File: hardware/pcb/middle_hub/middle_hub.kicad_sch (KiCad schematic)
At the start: 16 parts, among them J1 USB_A, J2 FH34SRJ-12S-0.5SH, J3 FH34SRJ-12S-0.5SH, J4 Conn_01x05, SW1 RotaryEncoder_Switch, U1 DT1446-04S, U2 AP2112K-3.3

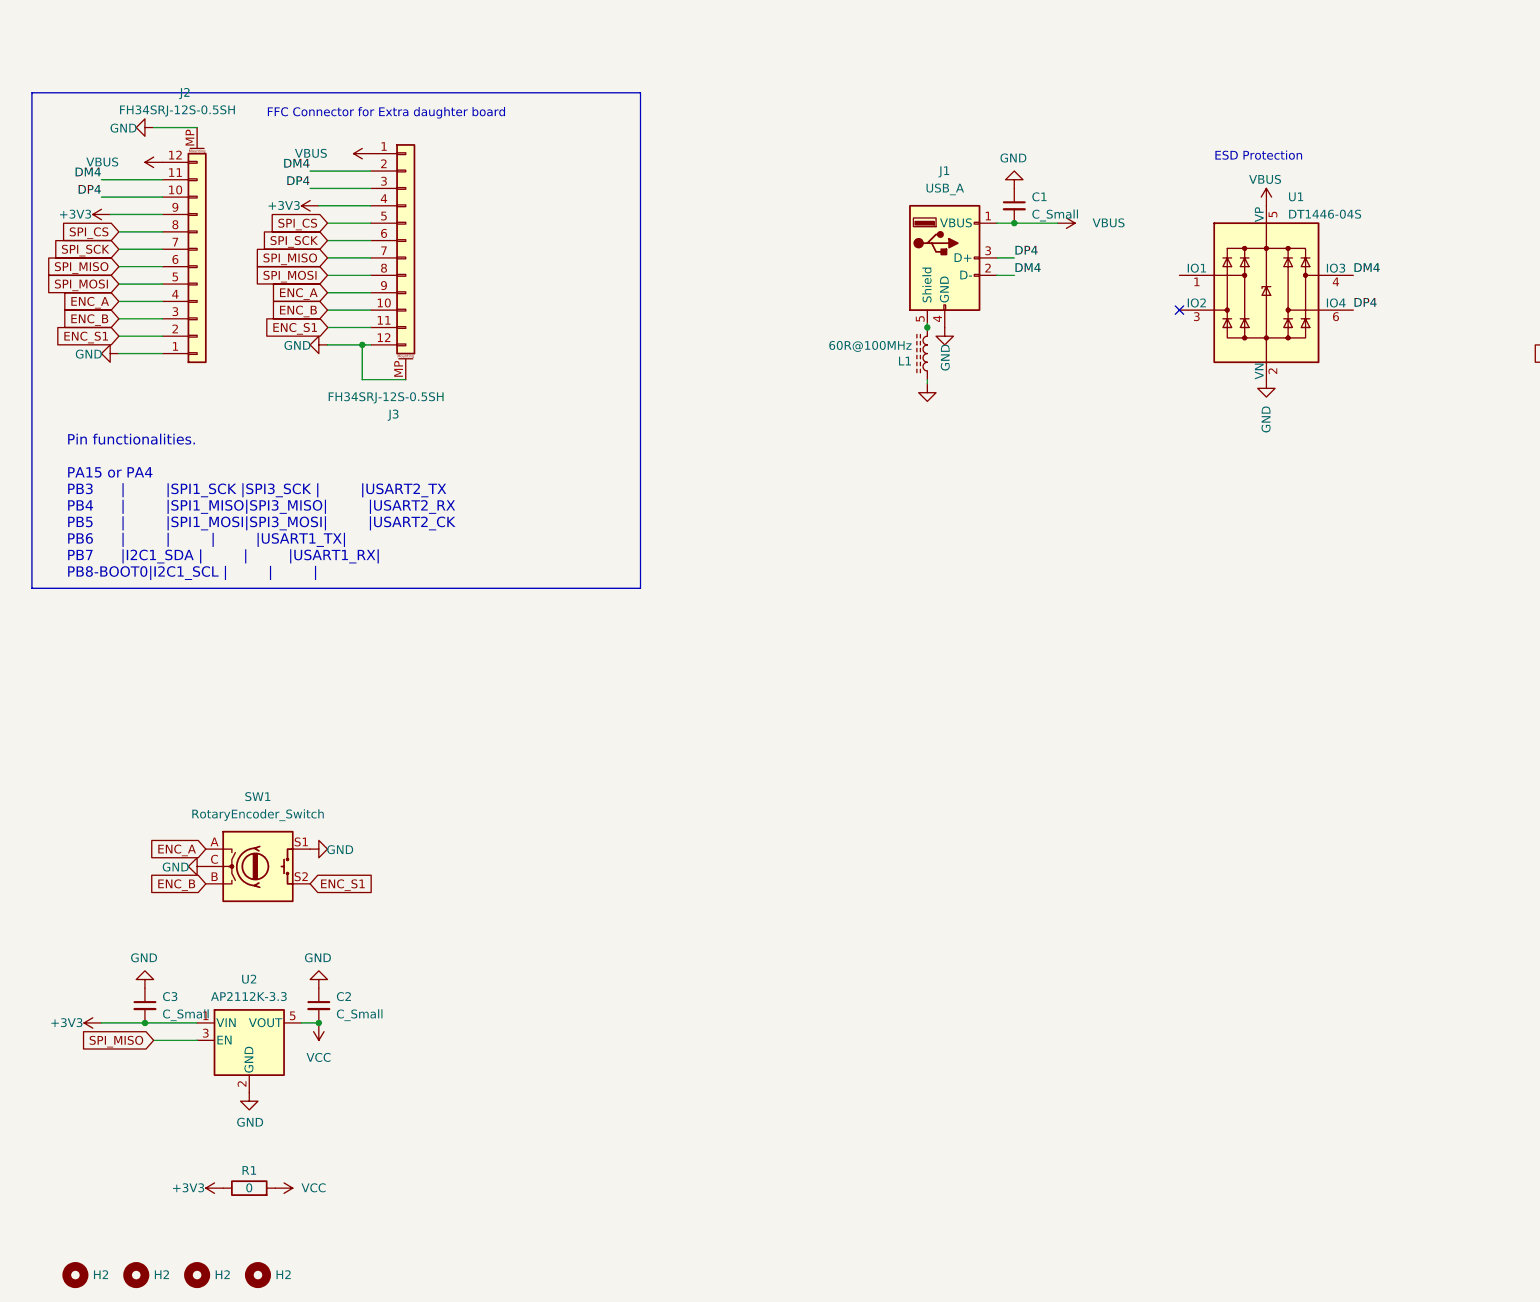
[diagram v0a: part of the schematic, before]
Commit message: preproduction
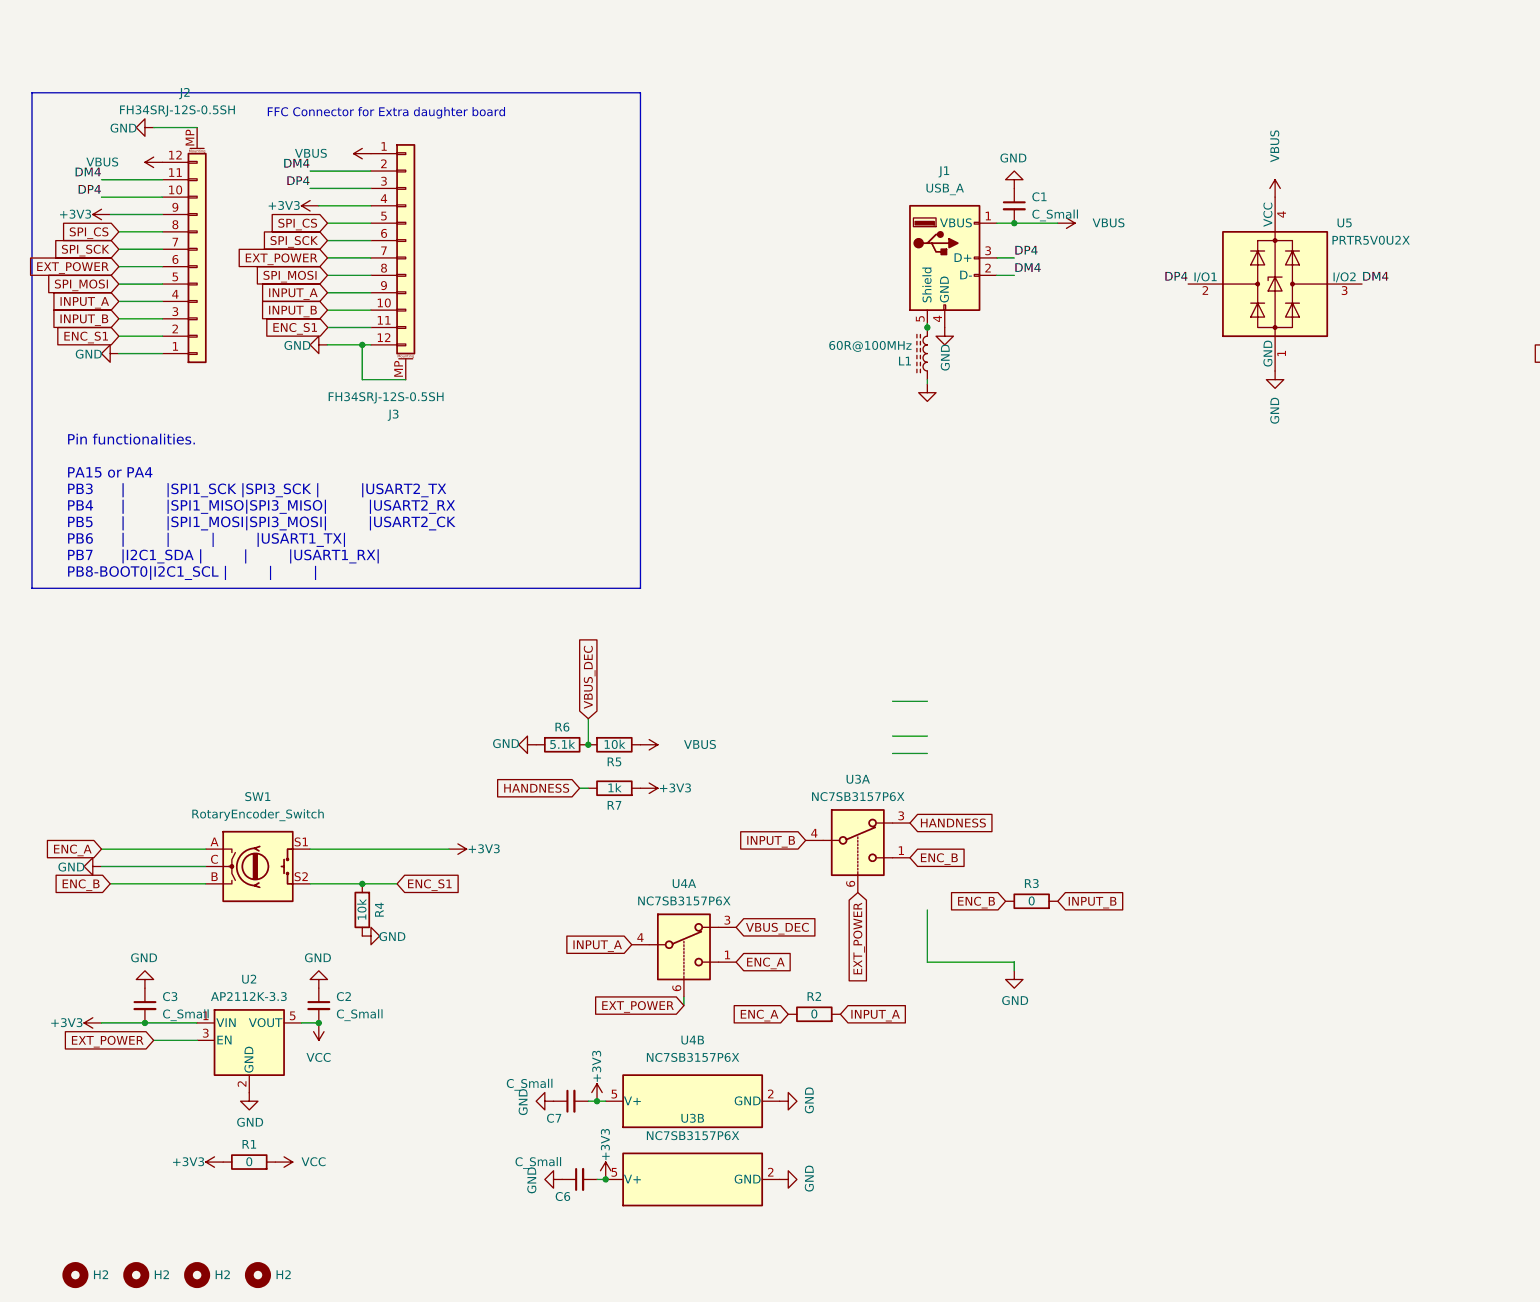
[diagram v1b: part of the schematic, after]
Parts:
- removed U1: DT1446-04S, PCM_Package_TO_SOT_SMD_AKL:SOT-363_SC-70-6_Handsoldering, symbol Power_Protection:SRV05-4
- added C6, C7: C_Small, PCM_Capacitor_SMD_AKL:C_0603_1608Metric_Pad1.05x0.95mm, symbol Device:C_Small
- added R2, R3: 0, PCM_Resistor_SMD_AKL:R_0402_1005Metric_Pad0.72x0.64mm_HandSolder, symbol Device:R
- added R4, R5: 10k, PCM_Resistor_SMD_AKL:R_0603_1608Metric, symbol Device:R
- added R6: 5.1k, PCM_Resistor_SMD_AKL:R_0603_1608Metric, symbol Device:R
- added R7: 1k, PCM_Resistor_SMD_AKL:R_0603_1608Metric, symbol Device:R
- added U3, U4: NC7SB3157P6X, PCM_Package_TO_SOT_SMD_AKL:SOT-363_SC-70-6_Handsoldering, symbol Analog_Switch:NC7SB3157P6X
- added U5: PRTR5V0U2X, PCM_Package_TO_SOT_SMD_AKL:SOT-143, symbol Power_Protection:PRTR5V0U2X
- R1: footprint PCM_Resistor_SMD_AKL:R_0603_1608Metric -> PCM_Resistor_SMD_AKL:R_0402_1005Metric_Pad0.72x0.64mm_HandSolder
- U2: footprint Package_TO_SOT_SMD:SOT-23-5 -> PCM_Package_TO_SOT_SMD_AKL:SOT-23-5
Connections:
- net +3V3: now also SW1.S1, C6.2, C7.2, R7.2, U3.5 (V+), U4.5 (V+)
- net DM4: now also U5.3 (I/O2)
- net DP4: now also U5.2 (I/O1)
- net ENC_A : now also R2.1, U4.1; no longer J2.4 (Pin_4), J3.9 (Pin_9)
- net ENC_B : now also R3.1, U3.1; no longer J2.3 (Pin_3), J3.10 (Pin_10)
- net ENC_S1: now also R4.2
- net GND: now also C6.1, C7.1, R4.1, R6.2, U3.2 (GND), U4.2 (GND), U5.1 (GND); no longer SW1.S1
- net VBUS: now also R5.1, U5.4 (VCC)
- net SPI_MISO renamed EXT_POWER
- net EXT_POWER: now also U3.6, U4.6
- new net HANDNESS: R7.1, U3.3
- new net INPUT_A: J2.4 (Pin_4), J3.9 (Pin_9), R2.2, U4.4
- new net INPUT_B: J2.3 (Pin_3), J3.10 (Pin_10), R3.2, U3.4
- new net VBUS_DEC: R5.2, R6.1, U4.3
- no-connect marks 2 -> 1
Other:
- note removed: "ESD Protection"
- moved on the sheet: R1

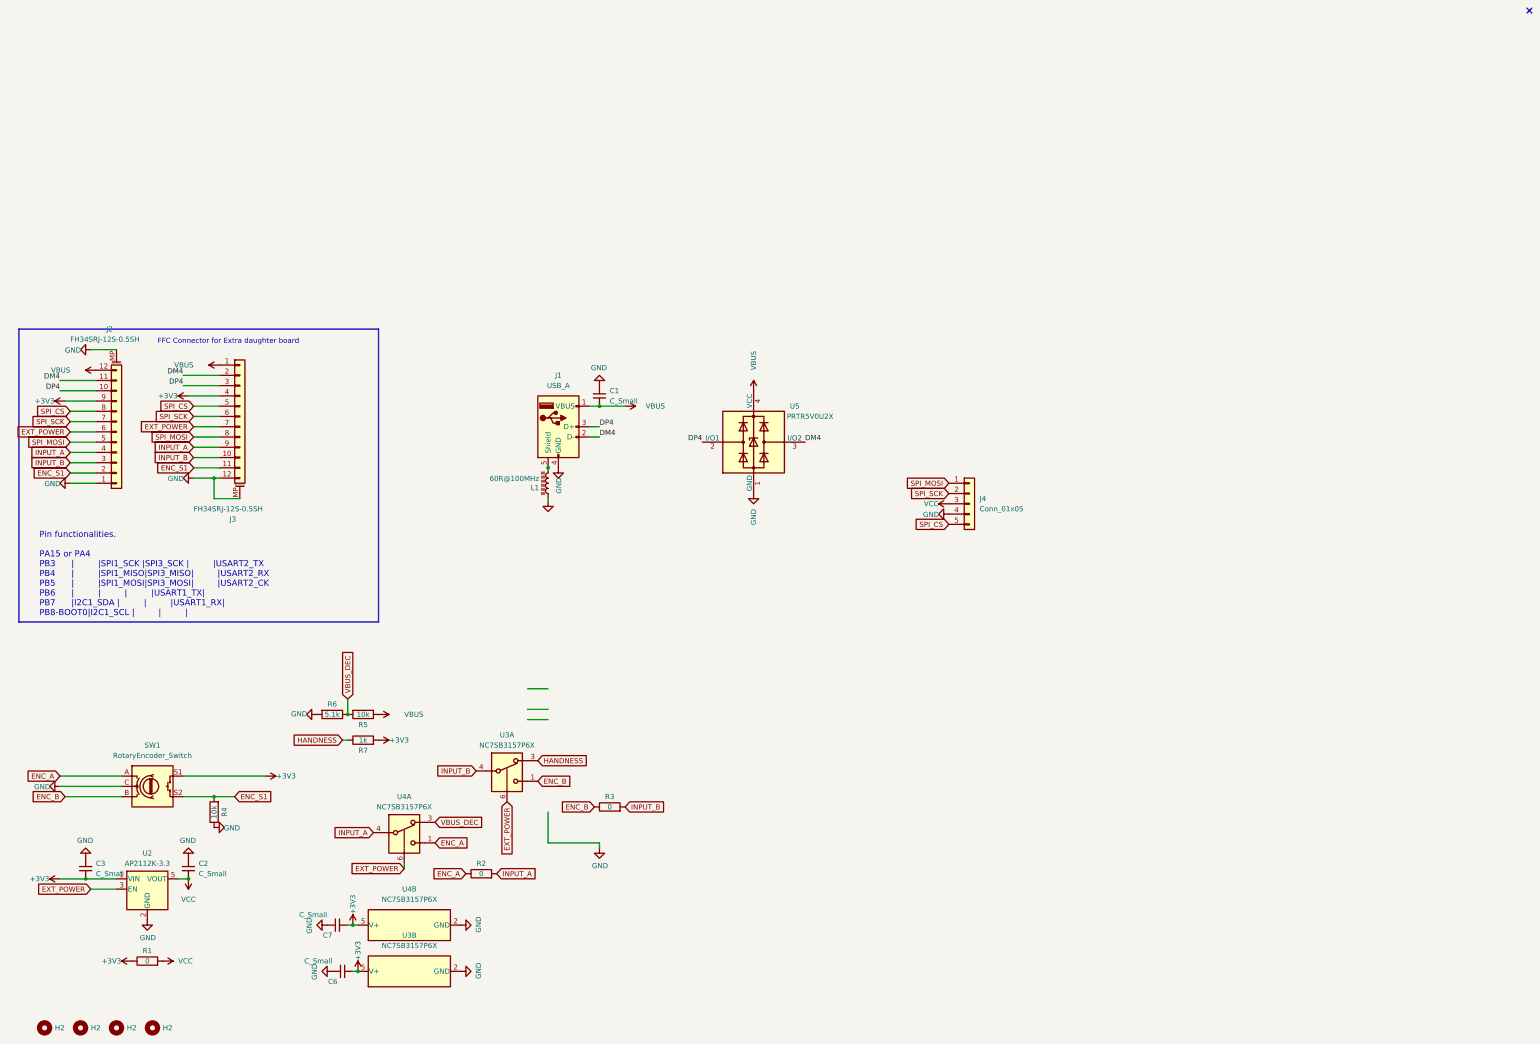
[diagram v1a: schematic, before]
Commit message: temp
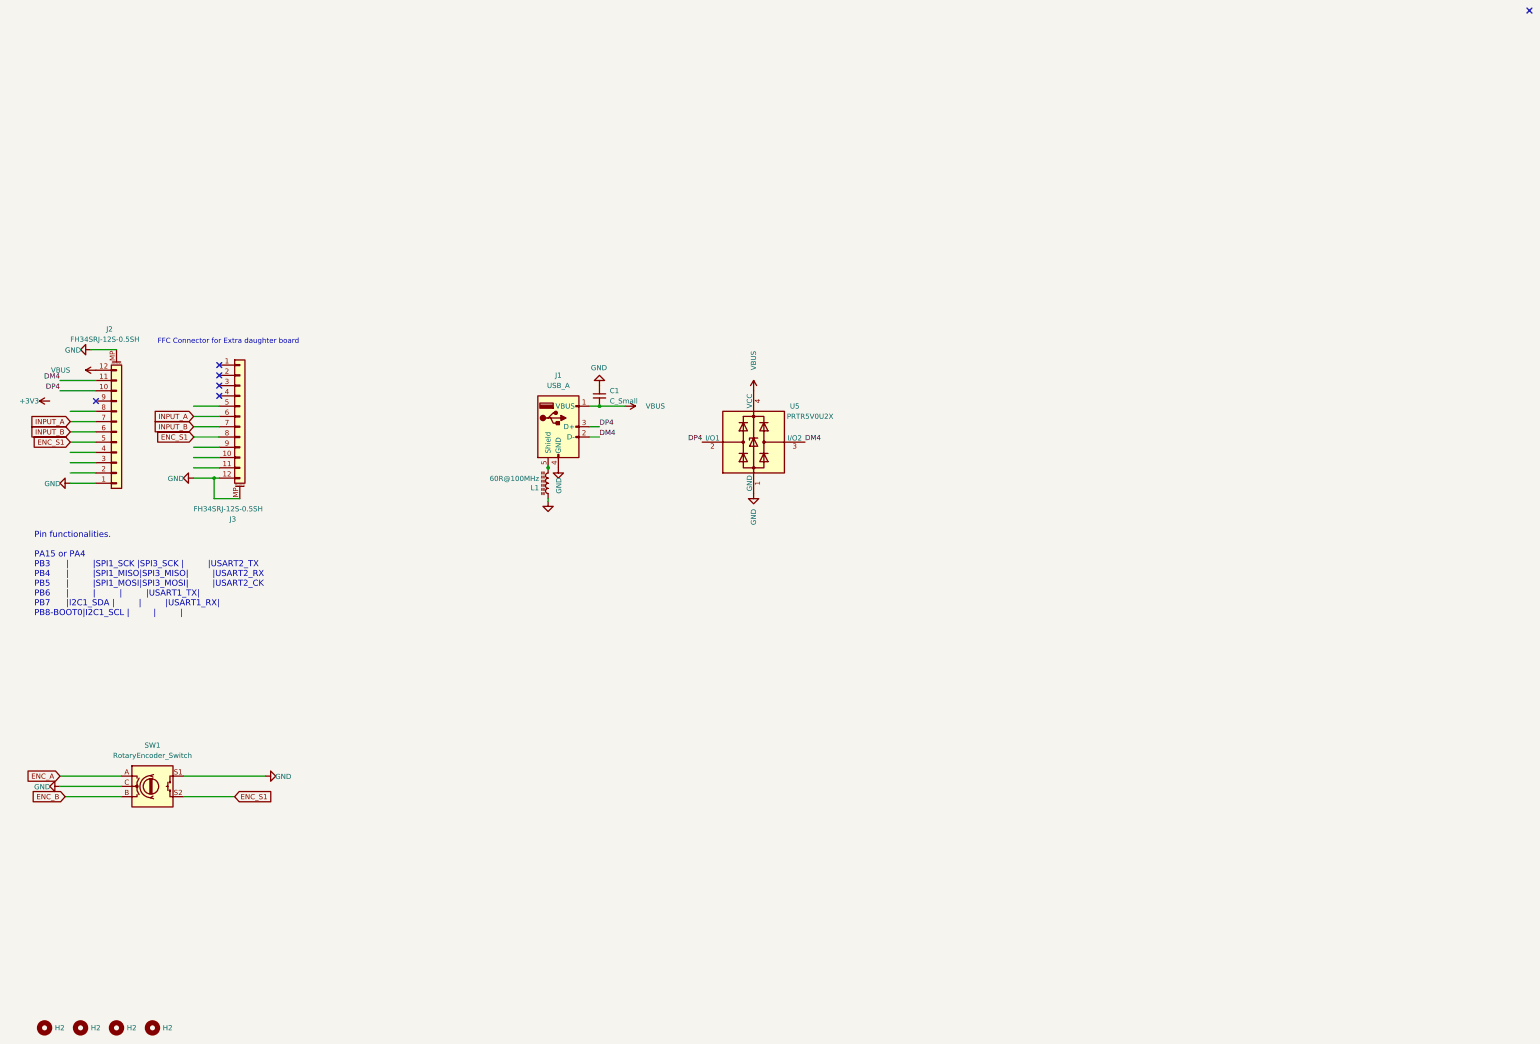
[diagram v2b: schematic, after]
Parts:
- removed C2, C3, C6, C7: C_Small, PCM_Capacitor_SMD_AKL:C_0603_1608Metric_Pad1.05x0.95mm, symbol Device:C_Small
- removed J4: Conn_01x05, ec_parts:NiceView_PinHeader_1x05_P2.54mm, symbol Connector_Generic:Conn_01x05
- removed R1, R2, R3: 0, PCM_Resistor_SMD_AKL:R_0402_1005Metric_Pad0.72x0.64mm_HandSolder, symbol Device:R
- removed R4, R5: 10k, PCM_Resistor_SMD_AKL:R_0603_1608Metric, symbol Device:R
- removed R6: 5.1k, PCM_Resistor_SMD_AKL:R_0603_1608Metric, symbol Device:R
- removed R7: 1k, PCM_Resistor_SMD_AKL:R_0603_1608Metric, symbol Device:R
- removed U2: AP2112K-3.3, PCM_Package_TO_SOT_SMD_AKL:SOT-23-5, symbol Regulator_Linear:AP2112K-3.3
- removed U3, U4: NC7SB3157P6X, PCM_Package_TO_SOT_SMD_AKL:SOT-363_SC-70-6_Handsoldering, symbol Analog_Switch:NC7SB3157P6X
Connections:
- net EXT_POWER is gone; now on net INPUT_B: J2.6 (Pin_6), J3.7 (Pin_7)
- net SPI_MOSI is gone; now on net ENC_S1: J2.5 (Pin_5), J3.8 (Pin_8)
- net SPI_SCK  is gone; now on net INPUT_A: J2.7 (Pin_7), J3.6 (Pin_6)
- net +3V3: no longer J2.9 (Pin_9), J3.4 (Pin_4), SW1.S1
- net DM4: no longer J3.2 (Pin_2)
- net DP4: no longer J3.3 (Pin_3)
- net ENC_S1: no longer J2.2 (Pin_2), J3.11 (Pin_11)
- net GND: now also SW1.S1
- net INPUT_A: no longer J2.4 (Pin_4), J3.9 (Pin_9)
- net INPUT_B: no longer J2.3 (Pin_3), J3.10 (Pin_10)
- net VBUS: no longer J3.1 (Pin_1)
- net SPI_CS  : no longer names the net of J3.5 (Pin_5)
- net SPI_CS  : no longer J2.8 (Pin_8)
- no-connect marks 1 -> 6
